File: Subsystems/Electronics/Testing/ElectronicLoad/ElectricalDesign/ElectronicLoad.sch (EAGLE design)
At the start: 51 parts, among them J1 USB, J2 Current Input, J3 Current Sense, J4 Voltage Sense, J5 SWD, Q1 IRFP4368PBF, Q2 SiRA20DP, Q3 SiRA20DP, Q4 IRFP4368PBF, U1 STM32L476RGT, U2 AD8515, U3 FT230XQ, U4 INA199C1, U5 STM32L476RGT, U6 INA199C1

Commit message: Update ElectronicLoad.sch
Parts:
- added C14, C15, C16, C17, C18, C21: 1µF 10%, CougsInSpace-Capacitors:CAP-H-1UF-1608
- added C19, C20: 1nF 1%, CougsInSpace-Capacitors:CAP-V-1NF-B-1608
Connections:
- removed net I_SENSE_IN+: J3.1, R2.2, U4.OUT, U5C.PC0
- new net A0_LCD: B1.A0, U5A.PA0
- new net CS_LCD: B1.!CS, U5A.PA2
- new net I_SENSE_IN: J3.1, R2.2, U4.OUT, U5C.PC0, U6.OUT
- new net N$10: B1.V3, C16.1
- new net N$11: B1.V4, C18.1
- new net N$2: B1.C1+, C20.1
- new net N$3: B1.C1-, C20.2
- new net N$4: B1.C2+, C19.1
- new net N$5: B1.C2-, C19.2
- new net N$6: B1.VOUT, C21.2
- new net N$7: B1.V0, C15.1
- new net N$8: B1.V1, C17.1
- new net N$9: B1.V2, C14.1
- new net RST_LCD: B1.!RST, U5A.PA1
- new net SPI_MOSI: B1.MOSI, U5A.PA7
- new net SPI_SCK: B1.SCK, U5A.PA5
- net AVDD: now also B1.LED+, B1.VDD
- net DGND: now also B1.LED-, B1.VSS, C14.2, C15.2, C16.2, C17.2, C18.2, C21.1
- net I_SENSE_IN-: no longer U6.OUT

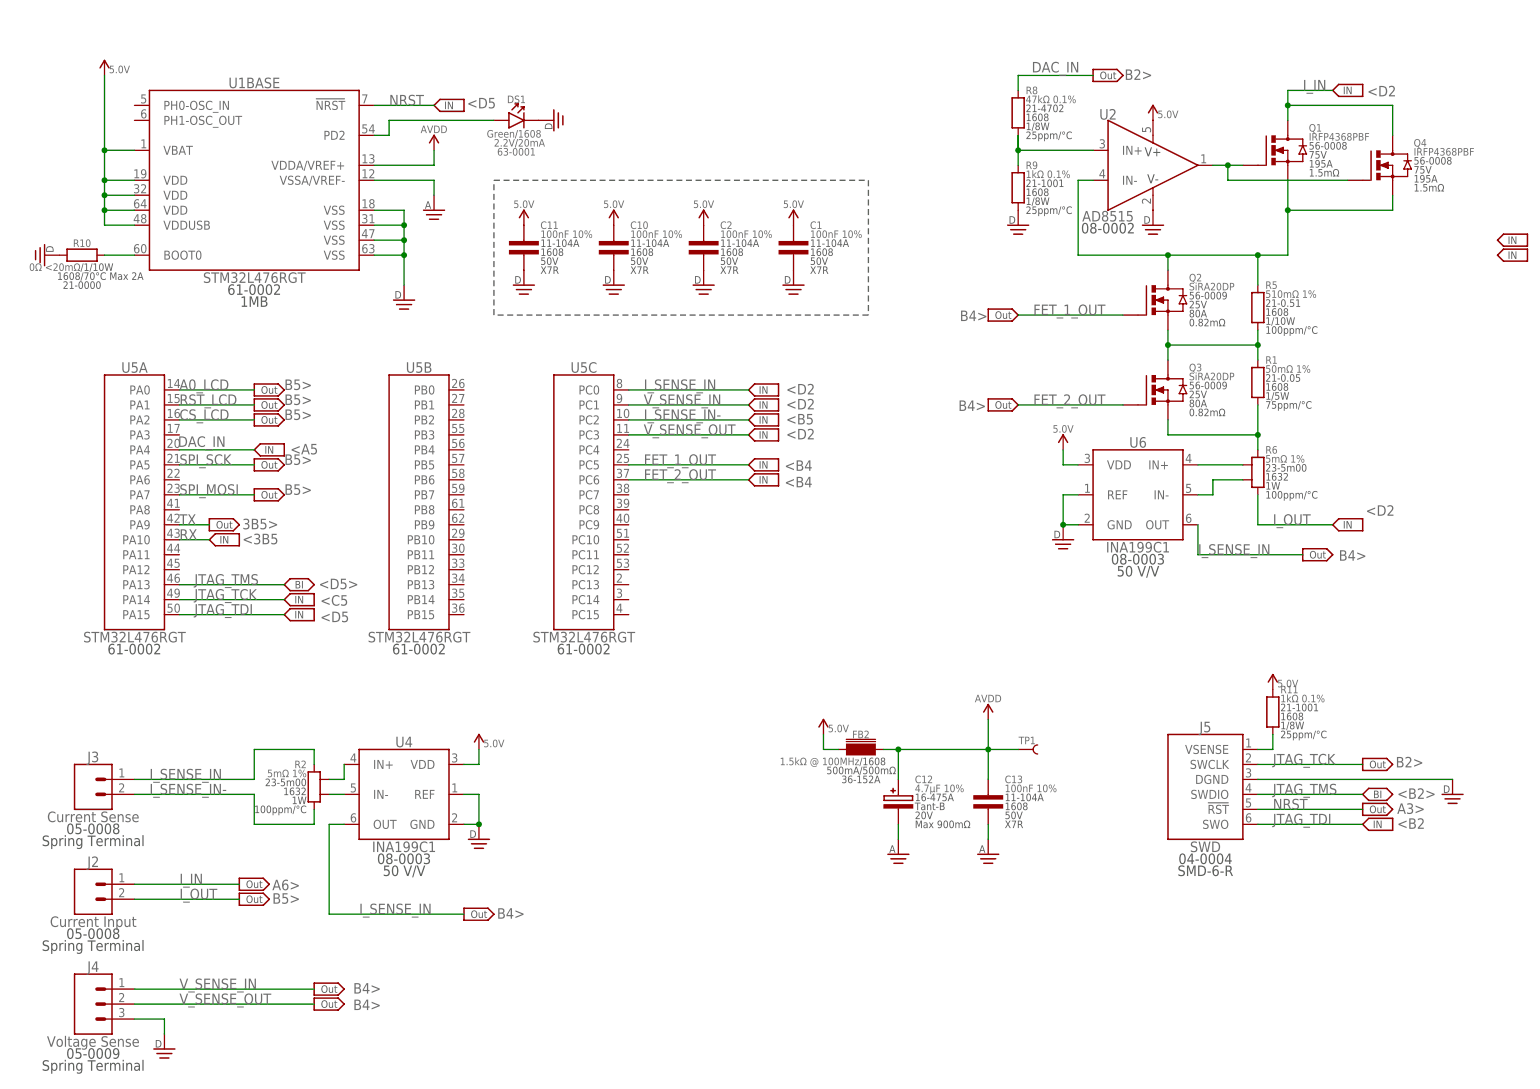
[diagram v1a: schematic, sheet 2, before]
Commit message: Update ElectronicLoad.sch
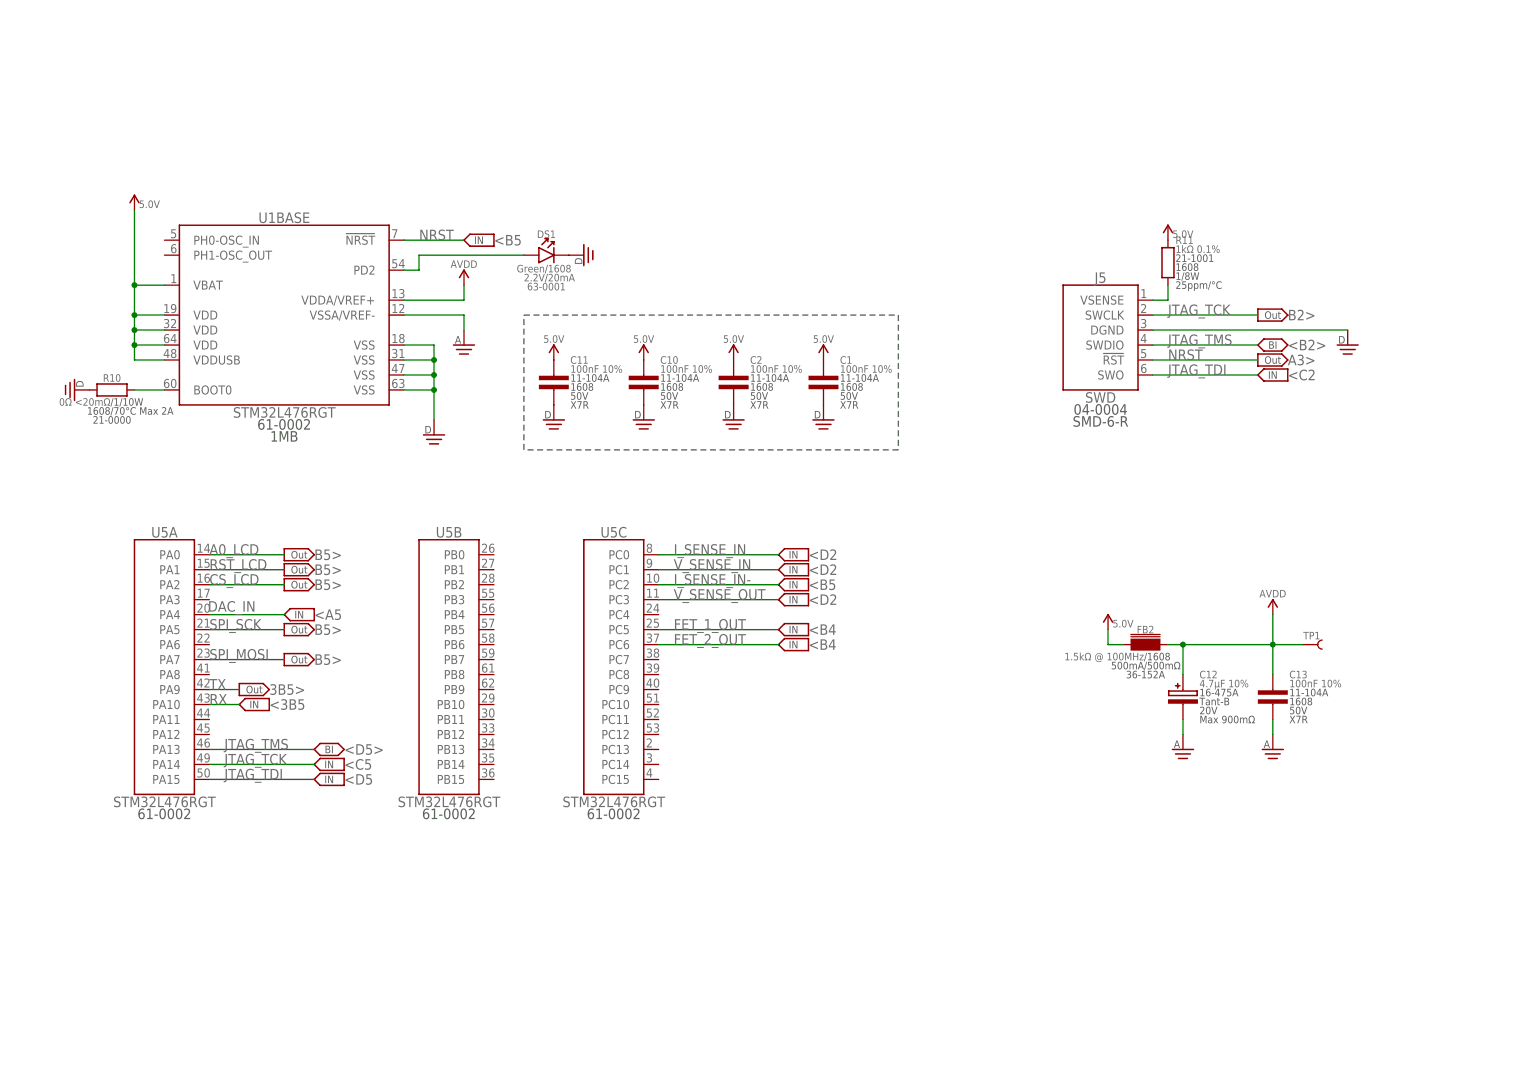
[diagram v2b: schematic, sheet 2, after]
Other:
- note added: "<C2"
- moved on the sheet: B1, C1, C10, C11, C12, C13, C14, C15, C16, C17, C18, C19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
